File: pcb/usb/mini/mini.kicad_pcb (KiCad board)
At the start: 2 copper layers, 50.8 x 25.4 mm, 2 parts, among them J1 USB_B_Mini, U1 CH340C

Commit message: Signed-off-by: Dmitry Ponyatov <dponyatov@samsa.local>
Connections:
- J1 pad 1: unconnected-(J1-Pad1) -> VCC5
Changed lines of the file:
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@@
   )
   (net 0 "")
-  (net 1 "unconnected-(J1-Pad1)")
+  (net 1 "VCC5")
   (net 2 "/D-")
   (net 3 "/D+")
@@
     (pad "" np_thru_hole circle (at -2.2 0 270) (size 0.9 0.9) (drill 0.9) (layers *.Cu *.Mask))
     (pad "1" smd rect (at -1.6 -2.6 270) (size 0.5 2.5) (layers "F.Cu" "F.Paste" "F.Mask")
-      (net 1 "unconnected-(J1-Pad1)") (pinfunction "VBUS") (pintype "power_out"))
+      (net 1 "VCC5") (pinfunction "VBUS") (pintype "power_out"))
     (pad "2" smd rect (at -0.8 -2.6 270) (size 0.5 2.5) (layers "F.Cu" "F.Paste" "F.Mask")
       (net 2 "/D-") (pinfunction "D-") (pintype "bidirectional"))

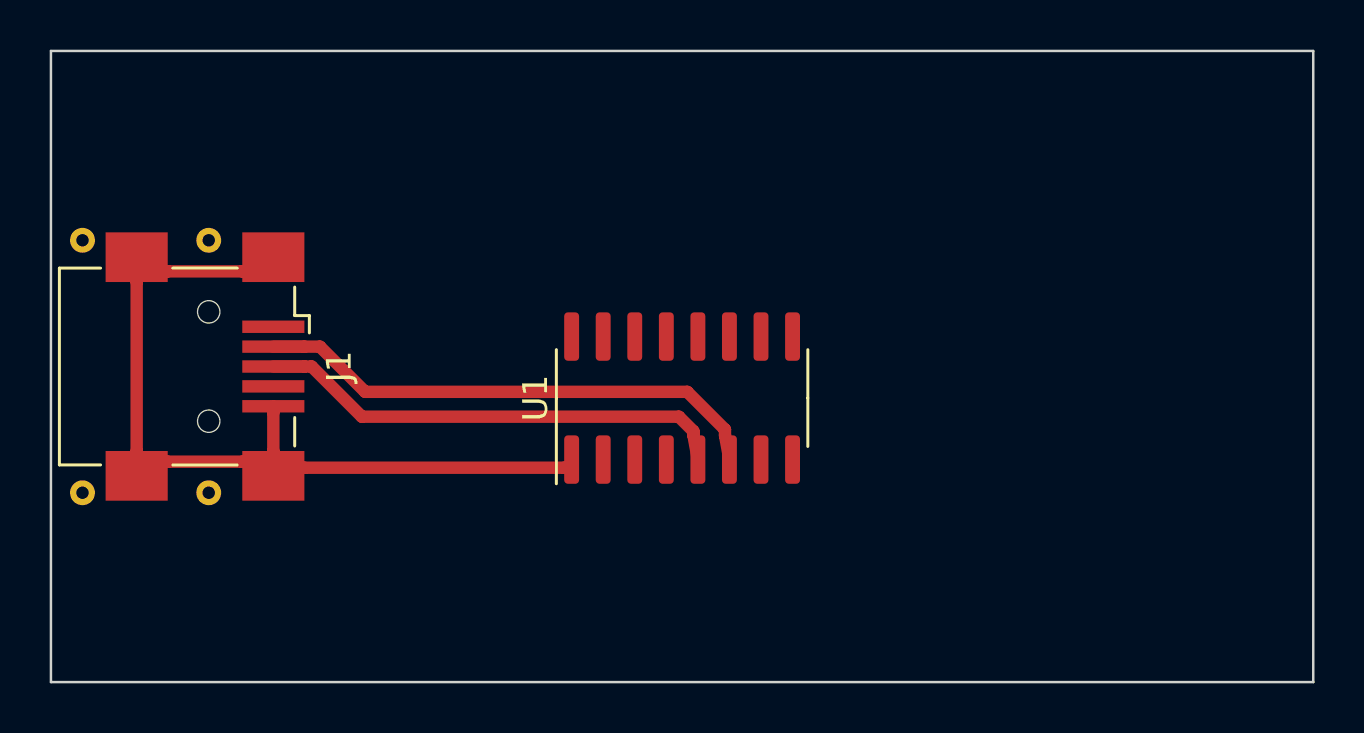
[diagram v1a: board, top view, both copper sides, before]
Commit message: Signed-off-by: Dmitry Ponyatov <dponyatov@samsa.local>
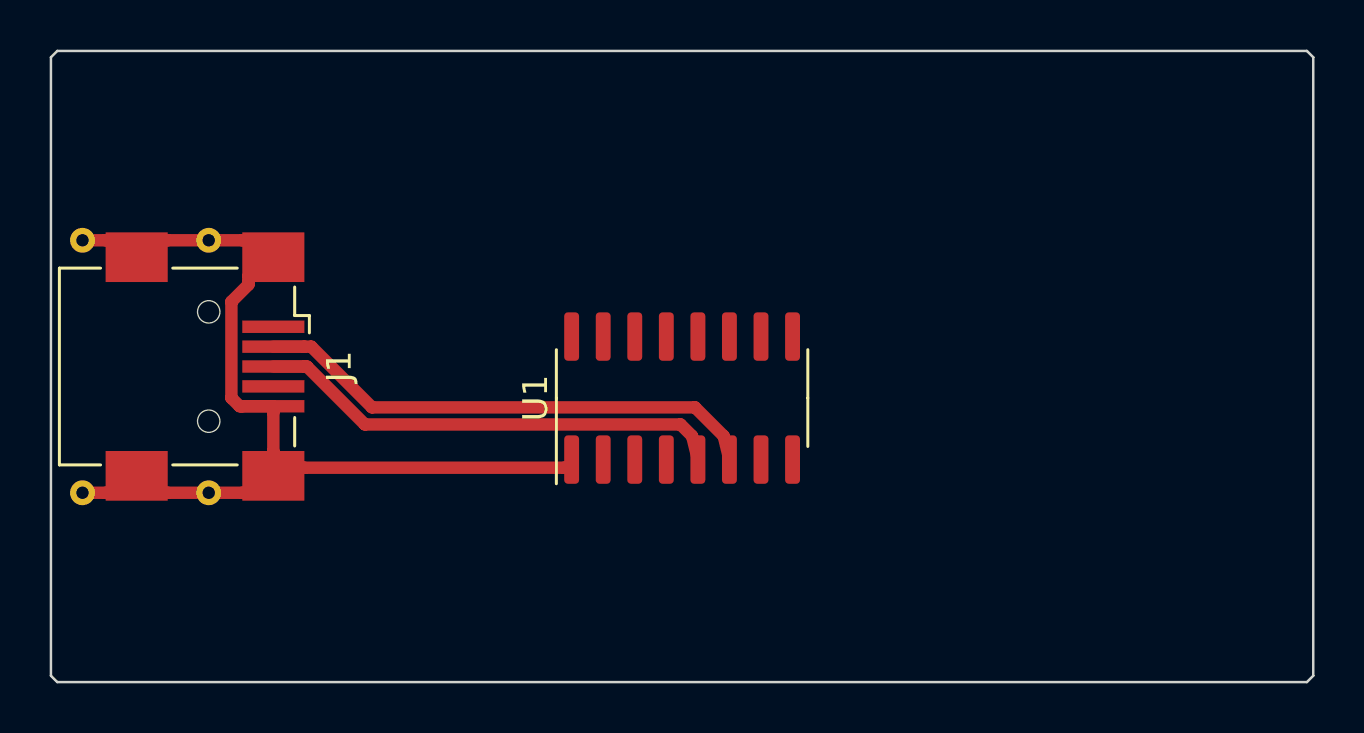
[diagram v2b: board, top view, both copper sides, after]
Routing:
- net GND: track 35.5 -> 40.0 mm
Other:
- outline, holes or cut-outs redrawn
